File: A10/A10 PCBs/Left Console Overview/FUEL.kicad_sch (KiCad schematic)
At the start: 31 parts, among them J1 FUEL, J2 FUEL ANALOG, SW1 L MAIN BOOST, SW10 L WING FILL DIS, SW11 L MAIN FILL DIS, SW12 FUEL RCVR, SW13 R WING FILL DIS, SW14 R MAIN FILL DIS, SW2 L WING BOOST, SW3 TK GATE, SW4 WING TANK, SW5 R MAIN BOOST, SW6 R WING BOOST, SW7 CROSS FEED, SW8 FUS EXT TANK, SW9 RCVR LTT OFF

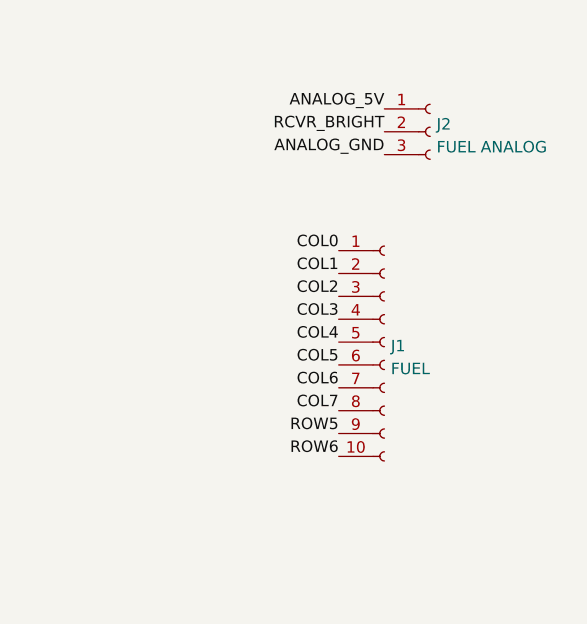
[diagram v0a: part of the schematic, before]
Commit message: A10
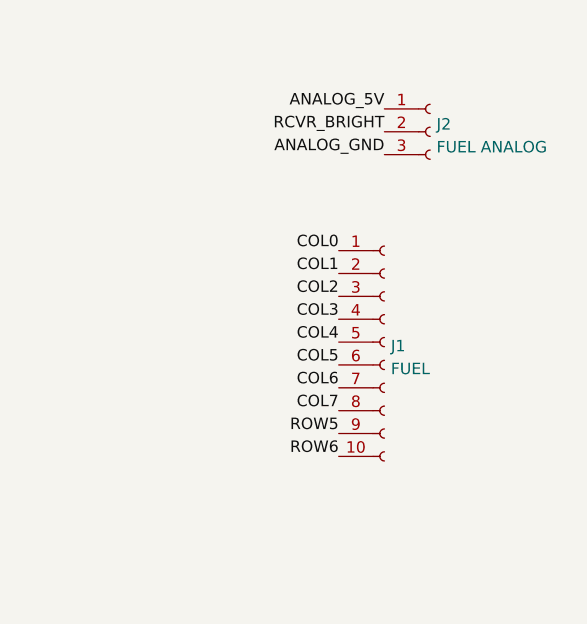
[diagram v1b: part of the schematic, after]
